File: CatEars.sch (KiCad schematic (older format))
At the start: 34 parts, among them J1 Conn_01x02_Male, J2 USB_B_Micro, J3 Conn_01x03, J4 Conn_01x01, J5 Conn_01x01, J6 Conn_01x01, J7 Conn_01x01, SW1 SW_Push, U1 ATSAMD21E18A-AU, U2 AP2112K-3.3

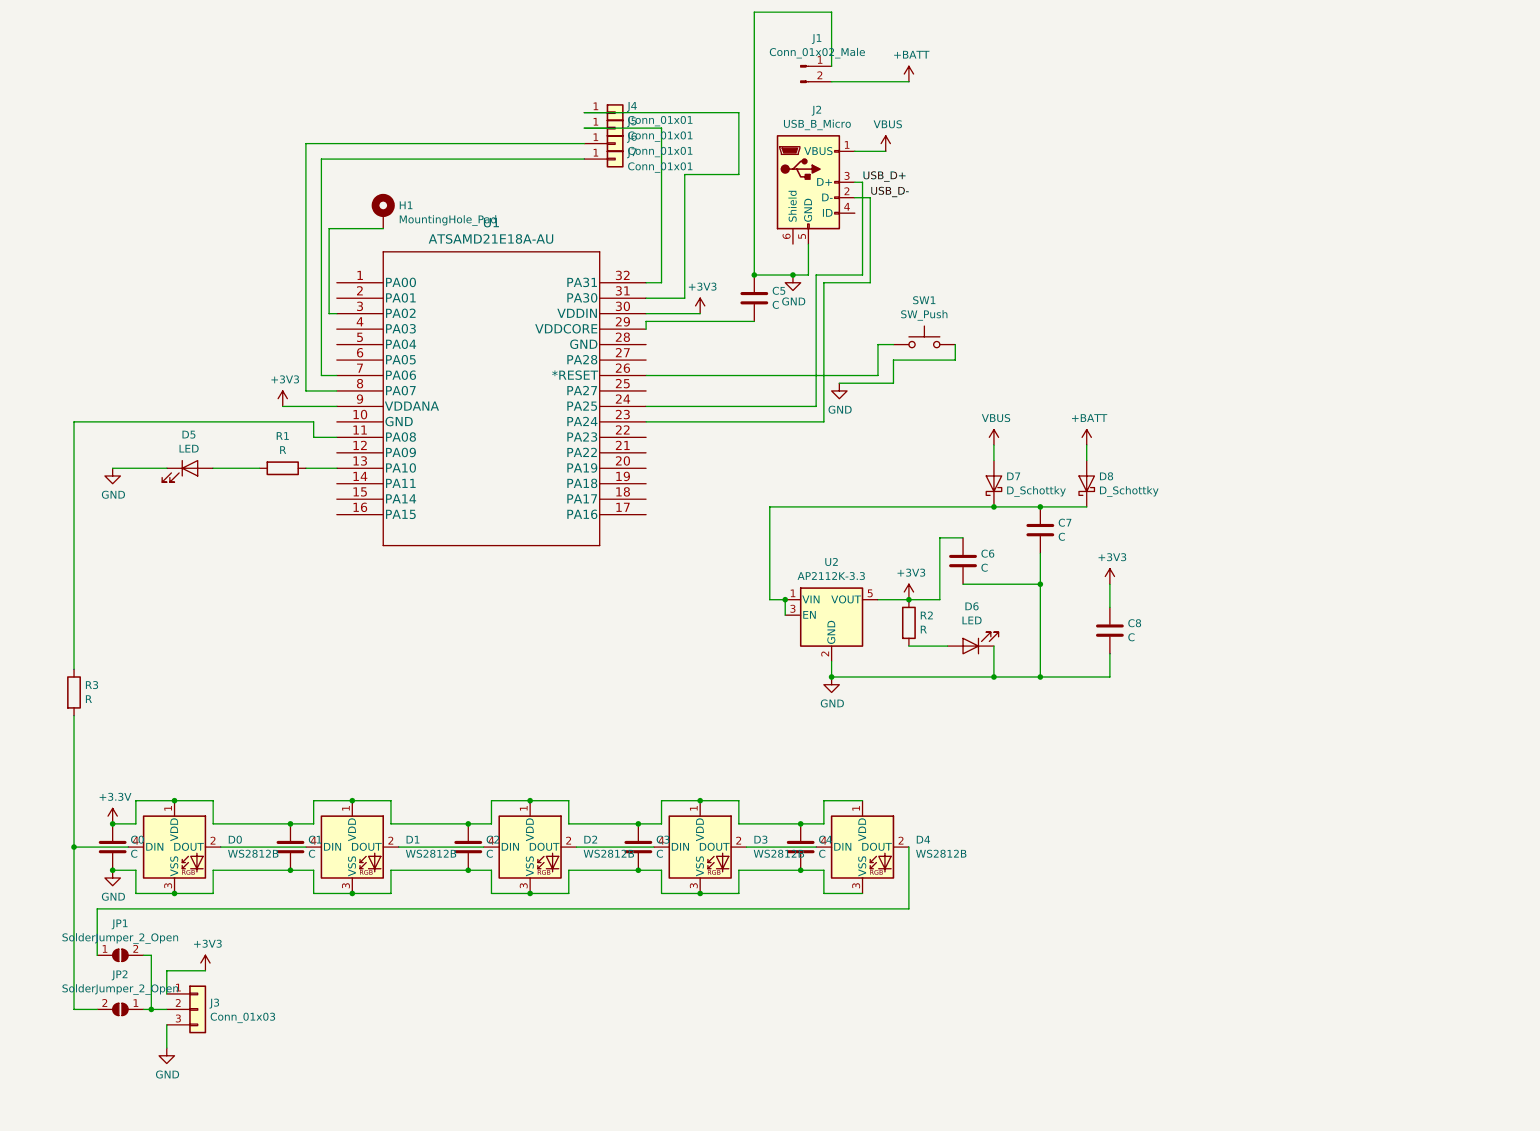
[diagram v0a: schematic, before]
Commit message: v3 PCB final + gerbers
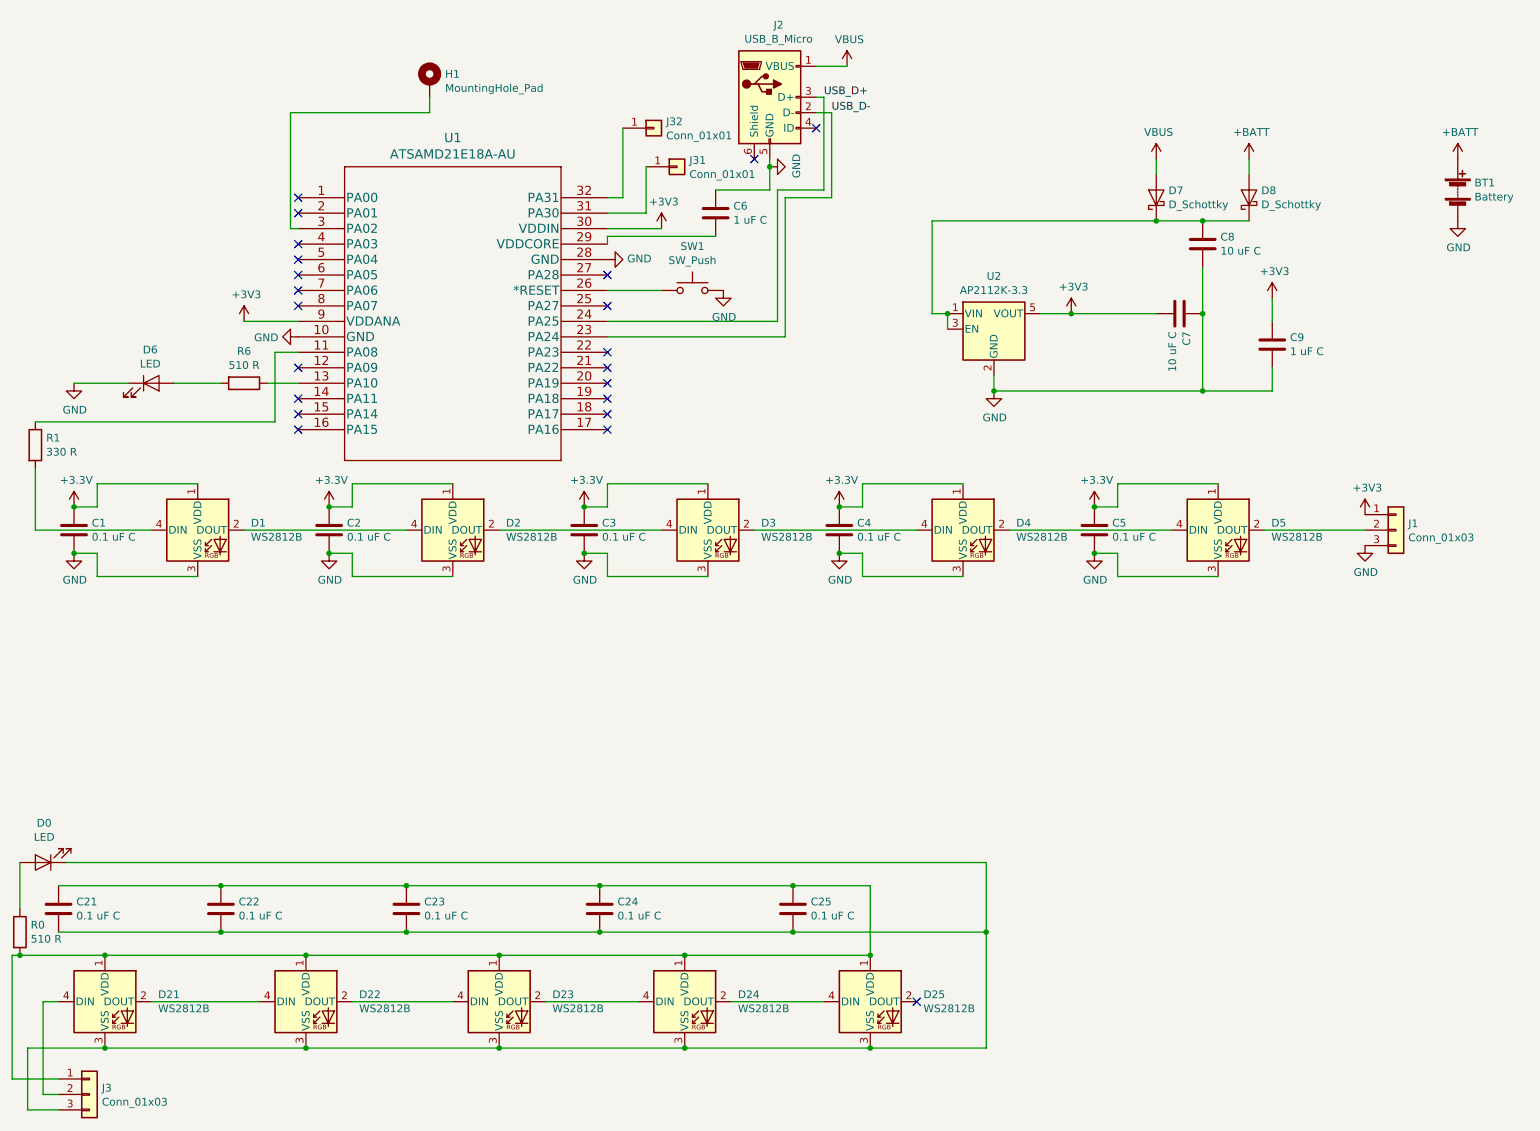
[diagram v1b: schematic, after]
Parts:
- removed C1: C, Capacitor_SMD:C_0603_1608Metric_Pad1.05x0.95mm_HandSolder, symbol Device:C
- removed D1: WS2812B, LED_SMD:LED_WS2812B_PLCC4_5.0x5.0mm_P3.2mm, symbol LED:WS2812B
- removed J1: Conn_01x02_Male, Connector_JST:JST_PH_B2B-PH-K_1x02_P2.00mm_Vertical, symbol Connector:Conn_01x02_Male
- removed J6, J7: Conn_01x01, TestPoint:TestPoint_Pad_D1.0mm, symbol Connector_Generic:Conn_01x01
- removed JP1, JP2: SolderJumper_2_Open, Jumper:SolderJumper-2_P1.3mm_Open_TrianglePad1.0x1.5mm, symbol Jumper:SolderJumper_2_Open
- added BT1: Battery, Connector_JST:JST_PH_S2B-PH-SM4-TB_1x02-1MP_P2.00mm_Horizontal, symbol Device:Battery
- added C21, C22, C23, C24, C25, C5: 0.1 uF C, Capacitor_SMD:C_0603_1608Metric_Pad1.05x0.95mm_HandSolder, symbol Device:C
- added D21, D22, D23, D24, D25, D5: WS2812B, LED_SMD:LED_WS2812B_PLCC4_5.0x5.0mm_P3.2mm, symbol LED:WS2812B
- added J3: Conn_01x03, Connector_PinSocket_2.54mm:PinSocket_1x03_P2.54mm_Vertical, symbol Connector_Generic:Conn_01x03
- C1: renamed from C0; value C -> 0.1 uF C
- C2, C3, C4: value C -> 0.1 uF C
- C6: renamed from C5; value C -> 1 uF C
- C7: renamed from C6; value C -> 10 uF C
- C8: renamed from C7; value C -> 10 uF C
- C9: renamed from C8; value C -> 1 uF C
- R0: renamed from R2; value R -> 510 R
- R1: renamed from R3; value R -> 330 R
- R6: renamed from R1; value R -> 510 R
- SW1: footprint Button_Switch_SMD:SW_SPST_TL3342 -> Button_Switch_SMD:SW_SPST_EVQPE1
- renumbered D6 to D0, D0 to D1, D5 to D6, J3 to J1, J4 to J31, J5 to J32
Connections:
- net +3V3: now also C7.2, C5.1, D5.1 (VDD); no longer C7.1, R0.1
- net +BATT: now also BT1.1 (+)
- net GND: now also C7.1, U1.10 (GND), U1.28 (GND), BT1.2 (-), C5.2, D5.3 (VSS); no longer C7.2, D0.1 (K)
- net at D1.2 (DOUT): now also D2.4 (DIN)
- net at D4.2 (DOUT): now also D5.4 (DIN)
- net at D0.2 (A): now also R0.1; no longer R0.2
- net at J1.2 (Pin_2): now also D5.2 (DOUT)
- new net: C21.2, C22.2, C23.2, C24.2, C25.2, D0.1 (K), D21.3 (VSS), D22.3 (VSS), D23.3 (VSS), D24.3 (VSS), D25.3 (VSS), J3.3 (Pin_3)
- new net: C21.1, C22.1, C23.1, C24.1, C25.1, D21.1 (VDD), D22.1 (VDD), D23.1 (VDD), D24.1 (VDD), D25.1 (VDD), J3.1 (Pin_1), R0.2
- new net: D21.2 (DOUT), D22.4 (DIN)
- new net: D21.4 (DIN), J3.2 (Pin_2)
- new net: D22.2 (DOUT), D23.4 (DIN)
- new net: D23.2 (DOUT), D24.4 (DIN)
- new net: D24.2 (DOUT), D25.4 (DIN)
- no-connect marks 0 -> 22
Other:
- moved on the sheet: C1, C6, C7, C8, C9, D0, D1, D6, D7, D8, H1, J1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
